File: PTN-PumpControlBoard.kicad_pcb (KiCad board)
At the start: 2 copper layers, 96 x 64 mm, 38 parts, among them J1 CAN_OUT, J2 CAN_IN, U1 PeripheralSOM, U2 EMC2305-1-AP-TR, U3 TLV6001DCK, U4 TLV6001DCK, U5 TLV6001DCK, U6 TLV6001DCK

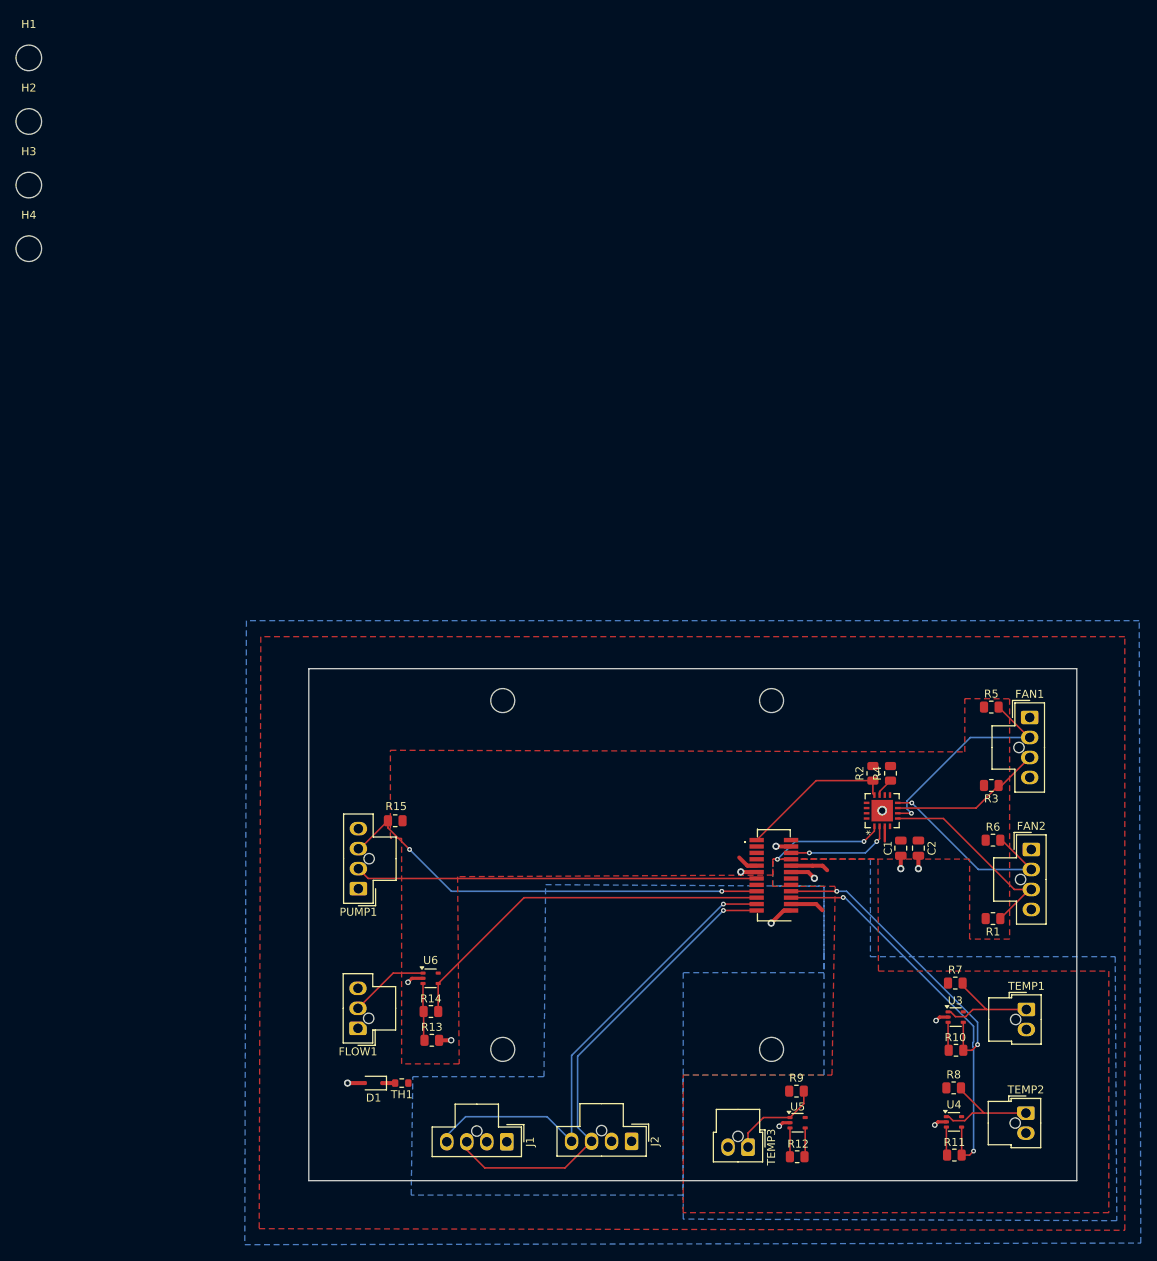
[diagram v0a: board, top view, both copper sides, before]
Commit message: added test points and headers, AGND and 12V not fully connected
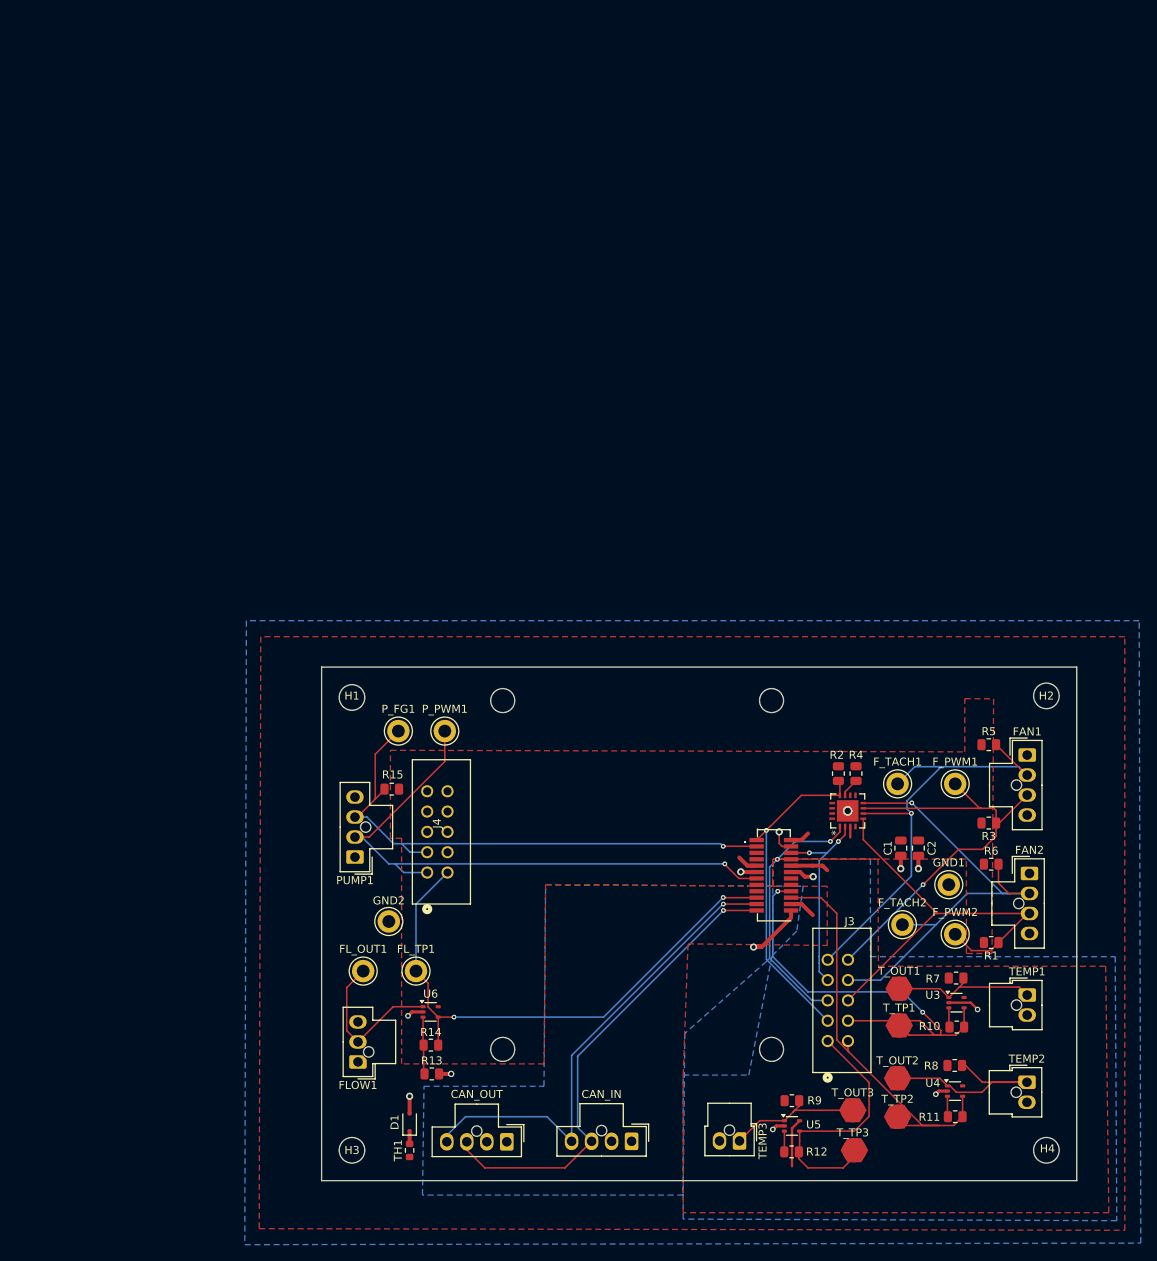
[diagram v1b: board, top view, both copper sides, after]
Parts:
- added FL_OUT1: Scope_TP, TestPoint:TestPoint_Keystone_5010-5014_Multipurpose, F.Cu at (62.8, 135.8)
- added FL_TP1: Scope_TP, TestPoint:TestPoint_Keystone_5010-5014_Multipurpose, F.Cu at (69.4, 135.8)
- added F_PWM1: Scope_TP, TestPoint:TestPoint_Keystone_5010-5014_Multipurpose, F.Cu at (136.8, 112.4)
- added F_PWM2: Scope_T1, TestPoint:TestPoint_Keystone_5010-5014_Multipurpose, F.Cu at (136.8, 131.2)
- added F_TACH1: Scope_TP, TestPoint:TestPoint_Keystone_5010-5014_Multipurpose, F.Cu at (129.6, 112.4)
- added F_TACH2: Scope_TP, TestPoint:TestPoint_Keystone_5010-5014_Multipurpose, F.Cu at (130.2, 130.0)
- added G***: LOGO, LOGO, F.Cu at (136.4, 158.6)
- added GND1: Scope_TP, TestPoint:TestPoint_Keystone_5010-5014_Multipurpose, F.Cu at (136.0, 125.0)
- added GND2: Scope_TP, TestPoint:TestPoint_Keystone_5010-5014_Multipurpose, F.Cu at (66.0, 129.6)
- added J3: SFH11-PBPC-D05-ST-BK, Headers:CONN_SFH11-xxxC-D05-ST-XX_SUL, F.Cu at (120.9, 144.5)
- added J4: SFH11-PBPC-D05-ST-BK, Headers:CONN_SFH11-xxxC-D05-ST-XX_SUL, F.Cu at (70.8, 123.5)
- added P_FG1: Scope_TP, TestPoint:TestPoint_Keystone_5010-5014_Multipurpose, F.Cu at (67.2, 105.8)
- added P_PWM1: Scope_TP, TestPoint:TestPoint_Keystone_5010-5014_Multipurpose, F.Cu at (73.0, 105.8)
- added T_OUT1: Pad_TP, UTSVT_Special:TestPoint_HEX_3mmID, F.Cu at (129.8, 138.0)
- added T_OUT2: Pad_TP, UTSVT_Special:TestPoint_HEX_3mmID, F.Cu at (129.6, 149.2)
- added T_OUT3: Pad_TP, UTSVT_Special:TestPoint_HEX_3mmID, F.Cu at (124.0, 153.2)
- added T_TP1: Pad_TP, UTSVT_Special:TestPoint_HEX_3mmID, F.Cu at (129.8, 142.6)
- added T_TP2: Pad_TP, UTSVT_Special:TestPoint_HEX_3mmID, F.Cu at (129.6, 154.0)
- added T_TP3: Pad_TP, UTSVT_Special:TestPoint_HEX_3mmID, F.Cu at (124.2, 158.2)
- moved H4 169.9 mm to (148.2, 158.2)
- moved H2 146.1 mm to (148.2, 101.4)
- moved H3 127.2 mm to (61.4, 158.2)
- moved H1 89.6 mm to (61.4, 101.6)
- moved TH1 8.47 mm to (68.6, 158.2), turned to 90 degrees
- moved D1 6.65 mm to (68.6, 154.7), turned to 90 degrees
- moved R11 4.80 mm to (136.8, 154.0)
- moved FAN1 4.71 mm to (145.8, 108.8)
- moved R3 4.71 mm to (141.0, 117.3)
- moved R5 4.71 mm to (141.0, 107.5)
- moved R2 4.31 mm to (122.2, 111.1)
- moved U2 4.31 mm to (123.4, 115.8)
- moved R4 4.31 mm to (124.4, 111.1)
- moved FLOW1 4.20 mm to (62.1, 147.2)
- moved R13 4.20 mm to (71.4, 148.7)
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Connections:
- U1 pad 17: /PUMP_FG -> unconnected-(U1-SPI1_MOSI-Pad17)
- U1 pad 3: unconnected-(U1-SPI2_MISO-Pad3) -> /PUMP_FG
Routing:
- net /FAN2_TACH: track 25.5 -> 61.2 mm
- net /FAN1_PWM: track 19.1 -> 54.7 mm, vias 0 -> 1
- net /FAN1_TACH: track 27.6 -> 59.5 mm
- net /TEMP3: track 3.64 -> 33.3 mm
- net /FAN2_PWM: track 25.7 -> 54.9 mm
- net /PUMP_PWM: track 50.3 -> 75.8 mm, vias 0 -> 1
- net /FLOW: track 47.7 -> 70.4 mm, vias 0 -> 2
- net /~{SMBALERT}: track 19.5 -> 41.9 mm, vias 0 -> 1
- net /TEMP1: track 38.5 -> 59.1 mm
- net /FAN_SCL: track 15.9 -> 33.8 mm
- net /PUMP_FG: track 55.4 -> 70.4 mm, vias 2 -> 1
- net /FAN_SDA: track 13.4 -> 25.5 mm
- net Net-(TEMP2-Pin_1): track 14.9 -> 26.7 mm
- net /FlowrateSensor/FLOW_OUT: track 9.95 -> 20.2 mm
- net Net-(TEMP3-Pin_1): track 11.8 -> 19.2 mm
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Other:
- board size 96 x 64 mm -> 94.4 x 64.2 mm
